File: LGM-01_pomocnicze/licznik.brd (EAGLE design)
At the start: 100 x 80 mm, 30 parts, among them IC1 7805L, J1 22-27-2041-04, Q3 BC557, T3 BC547, T4 BC547, T5 BC547

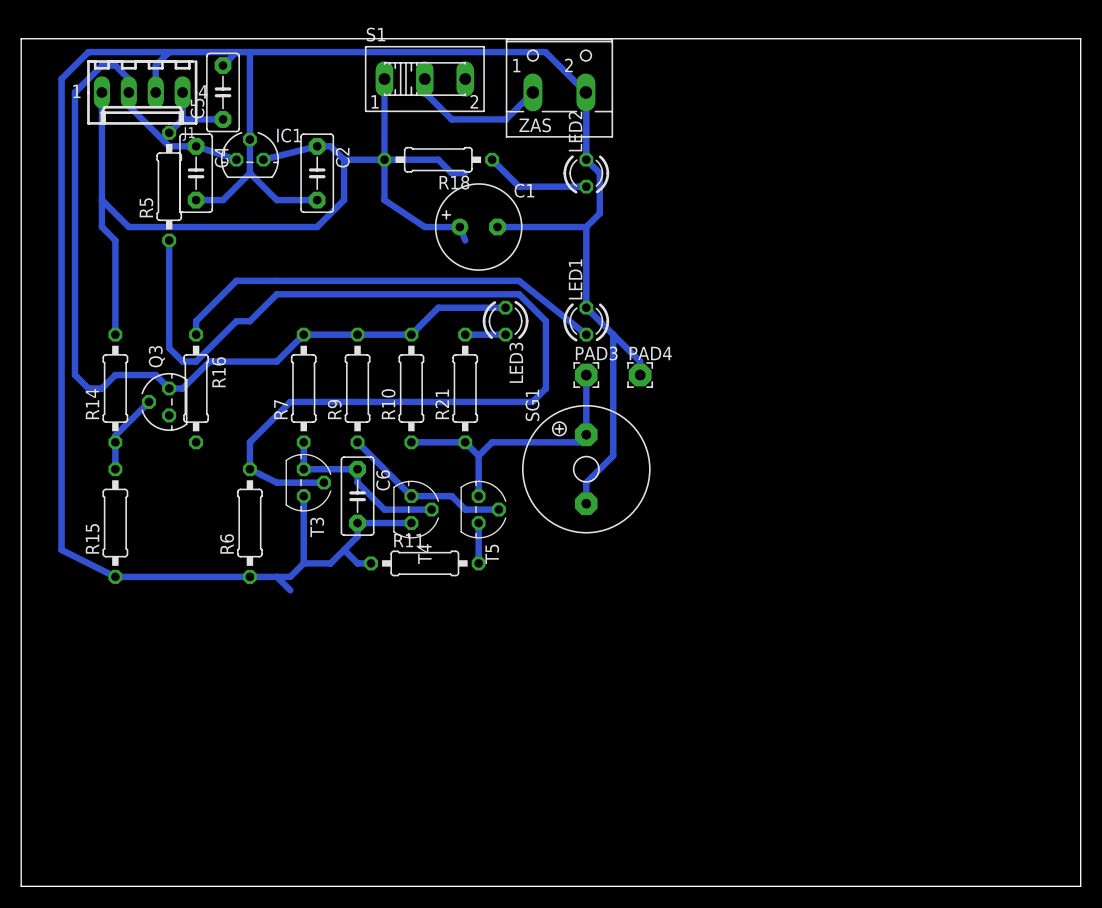
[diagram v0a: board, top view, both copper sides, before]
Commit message: Boards complete
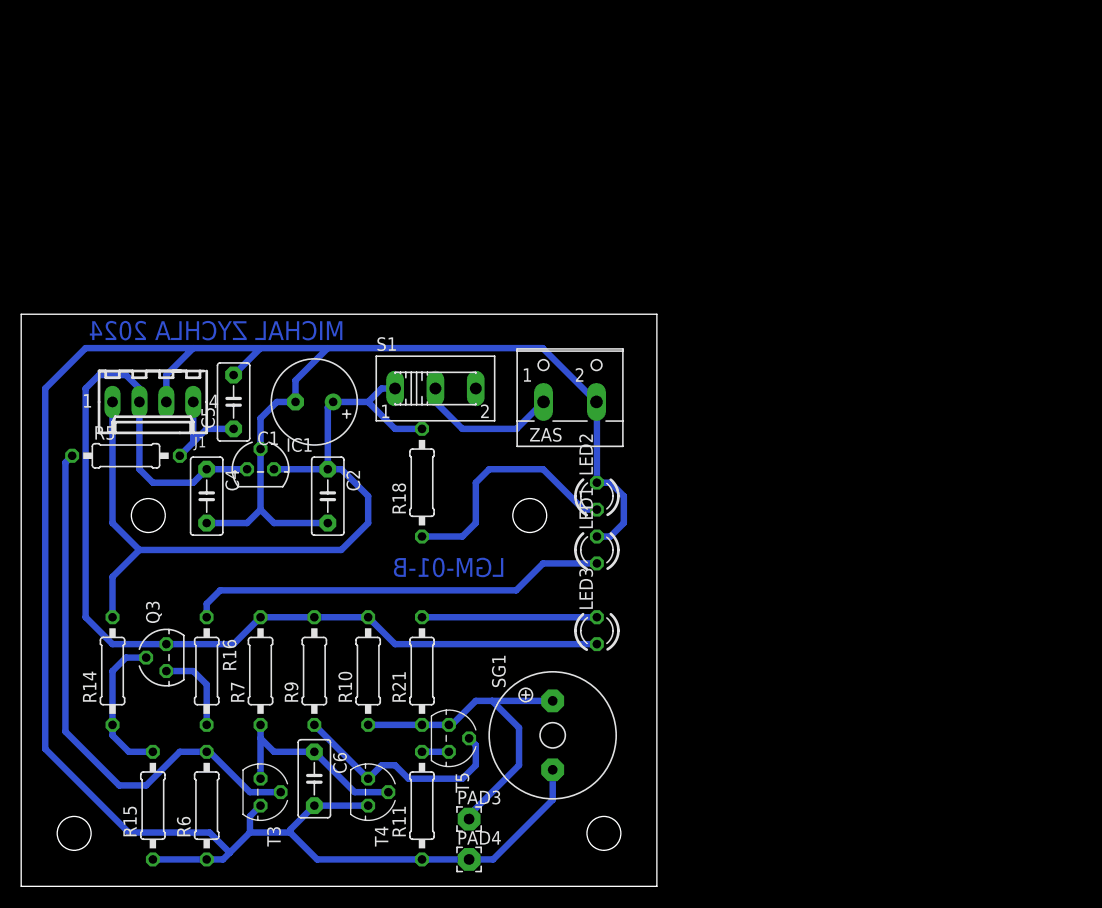
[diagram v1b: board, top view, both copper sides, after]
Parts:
- moved PAD4 48.5 mm to (42.3, 2.54)
- moved PAD3 43.3 mm to (42.3, 6.35)
- moved R18 30.5 mm to (37.8, 38.1), turned to 90 degrees
- moved C2 30.5 mm to (28.9, 36.8)
- moved C4 30.5 mm to (17.5, 36.8)
- moved LED2 30.5 mm to (54.3, 36.8)
- moved LED3 30.5 mm to (54.3, 24.1), turned to 90 degrees
- moved T3 29.5 mm to (22.6, 8.89)
- moved C5 29.2 mm to (20.1, 45.7)
- moved J1 29.2 mm to (12.4, 45.7)
- moved IC1 29.2 mm to (22.6, 39.4)
- moved S1 29.2 mm to (39.1, 47.0)
- moved ZAS 29.2 mm to (51.8, 47.0)
- moved R10 27.0 mm to (32.8, 20.3)
- moved R21 27.0 mm to (37.8, 20.3)
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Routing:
- net N$17: track 96.1 -> 51.6 mm
- net VBAT: track 93.1 -> 76.6 mm
- net N$14: track 9.94 -> 23.0 mm
- net N$24: track 3.81 -> 16.5 mm
- net N$22: track 0.00 -> 8.15 mm
- net N$23: track 7.67 -> 14.2 mm
- net N$21: track 16.0 -> 21.7 mm
- net GND: track 230.6 -> 225.1 mm
- net +5V: track 93.2 -> 98.0 mm
- net WYJSCIE: track 28.0 -> 32.5 mm
- net N$18: track 16.9 -> 19.2 mm
- net KATODA: track 8.15 -> 9.94 mm
- net N$15: track 41.5 -> 39.7 mm
- net N$19: track 3.81 -> 2.54 mm
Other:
- board size 100 x 80 mm -> 60 x 54 mm
- board text added: "LGM-01-B"
- board text added: "MICHAL ZYCHLA 2024"
